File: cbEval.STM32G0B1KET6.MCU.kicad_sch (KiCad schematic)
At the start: 20 parts, among them J10 Bergstik-II_6, J11 Bergstik-II_6, J12 Bergstik-II_8, J13 Bergstik-II_6, J14 CNC-Tech 2x5, U1 STM32G0B1KET6, Y1 16.000MHz

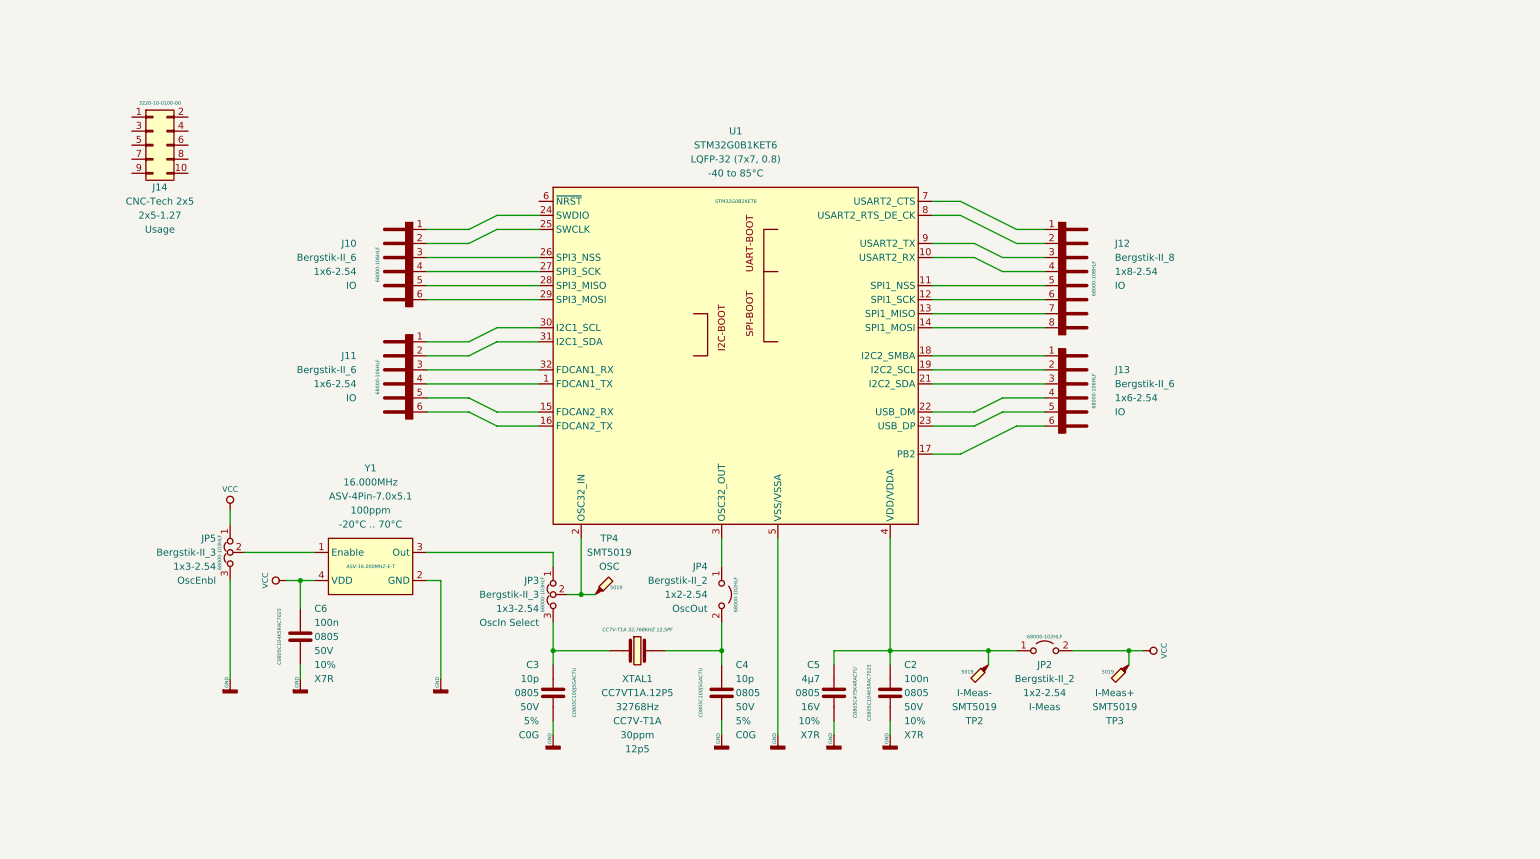
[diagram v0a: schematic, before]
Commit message: Zwischenstand (Sicherung)
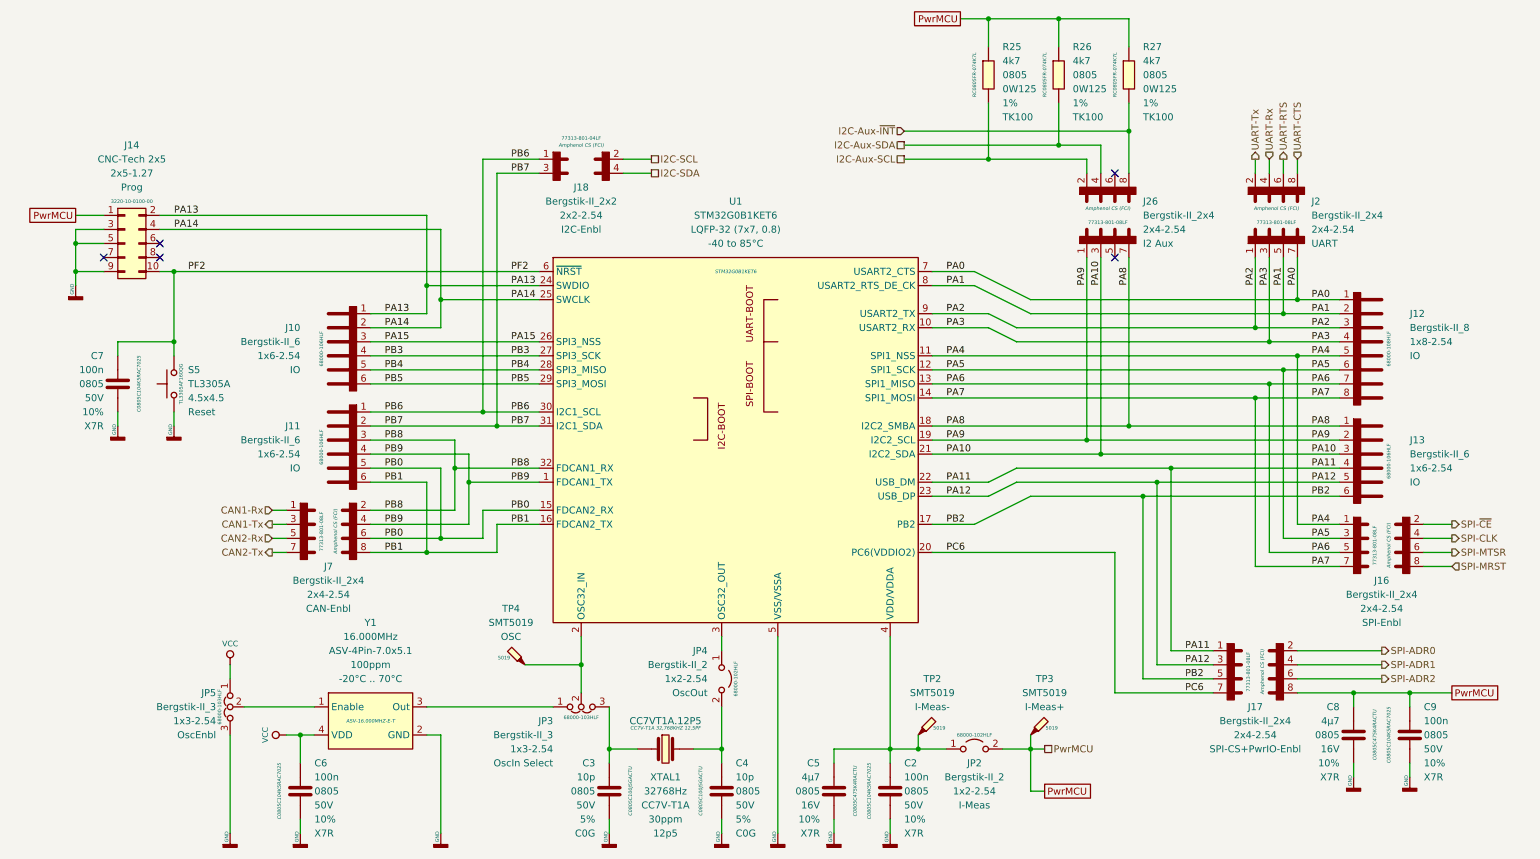
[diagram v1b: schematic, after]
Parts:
- added C7, C9: 100n, Capacitor_SMD:C_0805_2012Metric, symbol C.Kemet.MLCC.0805.X7R:100n
- added C8: 4µ7, Capacitor_SMD:C_0805_2012Metric, symbol C.Kemet.MLCC.0805.X7R:4µ7
- added J16, J17, J2, J26, J7: Bergstik-II_2x4, Connector_PinHeader_2.54mm:PinHeader_2x04_P2.54mm_Vertical, symbol J.PinHeader:Bergstik-II_2x4
- added J18: Bergstik-II_2x2, Connector_PinHeader_2.54mm:PinHeader_2x02_P2.54mm_Vertical, symbol J.PinHeader:Bergstik-II_2x2
- added R25, R26, R27: 4k7, Resistor_SMD:R_0805_2012Metric, symbol R.Yageo.RC0805:4k7
- added S5: TL3305A, Button_Switch_SMD:SW_SPST_TL3305A, symbol S:TL3305A
- J14: Usage Usage -> Prog
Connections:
- net GND: now also J14.3 (Pin_3), J14.5 (Pin_5), J14.9 (Pin_9), C7.2, C8.2, C9.2, S5.2
- net VCC: no longer JP2.2 (B), TP3.1
- net PA0: now reaches J12.1 (A1), U1.7 (USART2_CTS)
- net PA0: now also J2.7 (A4)
- net PA1: now reaches J12.2 (A2), U1.8 (USART2_RTS_DE_CK)
- net PA1: now also J2.5 (A3)
- net PA2: now reaches J12.3 (A3), U1.9 (USART2_TX)
- net PA2: now also J2.1 (A1)
- net PA3: now reaches J12.4 (A4), U1.10 (USART2_RX)
- net PA3: now also J2.3 (A2)
- net PA4: now reaches J12.5 (A5), U1.11 (SPI1_NSS)
- net PA4: now also J16.1 (A1)
- net PA5: now reaches J12.6 (A6), U1.12 (SPI1_SCK)
- net PA5: now also J16.3 (A2)
- net PA6: now reaches J12.7 (A7), U1.13 (SPI1_MISO)
- net PA6: now also J16.5 (A3)
- net PA7: now reaches J12.8 (A8), U1.14 (SPI1_MOSI)
- net PA7: now also J16.7 (A4)
- net PwrMCU: now reaches J14.1 (Pin_1)
- net PwrMCU: now also JP2.2 (B), TP3.1, C8.1, C9.1, J17.8 (B4), R25.1, R26.1, R27.1
- net PF2: now reaches J14.10 (Pin_10)
- net PF2: now also U1.6 (~{NRST}), C7.1, S5.1
- net PA13: now reaches J14.2 (Pin_2)
- net PA13: now also J10.1 (A1), U1.24 (SWDIO)
- net PA14: now reaches J14.4 (Pin_4)
- net PA14: now also J10.2 (A2), U1.25 (SWCLK)
- net PB9: now reaches J11.4 (A4), U1.1 (FDCAN1_TX)
- net PB9: now also J7.4 (B2)
- net PB0: now reaches J11.5 (A5), U1.15 (FDCAN2_RX)
- net PB0: now also J7.6 (B3)
- net PB1: now reaches J11.6 (A6), U1.16 (FDCAN2_TX)
- net PB1: now also J7.8 (B4)
- net PB2: now reaches J13.6 (A6), U1.17 (PB2)
- net PB2: now also J17.5 (A3)
- net PA8: now reaches J13.1 (A1), U1.18 (I2C2_SMBA)
- net PA8: now also J26.7 (A4)
- net PA9: now reaches J13.2 (A2), U1.19 (I2C2_SCL)
- net PA9: now also J26.1 (A1)
- net PA10: now reaches J13.3 (A3), U1.21 (I2C2_SDA)
- net PA10: now also J26.3 (A2)
- net PA11: now reaches J13.4 (A4), U1.22 (USB_DM)
- net PA11: now also J17.1 (A1)
- net PA12: now reaches J13.5 (A5), U1.23 (USB_DP)
- net PA12: now also J17.3 (A2)
- net PA15: now reaches J10.3 (A3), U1.26 (SPI3_NSS)
- net PB3: now reaches J10.4 (A4), U1.27 (SPI3_SCK)
- net PB4: now reaches J10.5 (A5), U1.28 (SPI3_MISO)
- net PB5: now reaches J10.6 (A6), U1.29 (SPI3_MOSI)
- net PB6: now reaches J11.1 (A1), U1.30 (I2C1_SCL)
- net PB6: now also J18.1 (A1)
- net PB7: now reaches J11.2 (A2), U1.31 (I2C1_SDA)
- net PB7: now also J18.3 (A2)
- net PB8: now reaches J11.3 (A3), U1.32 (FDCAN1_RX)
- net PB8: now also J7.2 (B1)
- new net CAN1-Rx: J7.1 (A1)
- new net CAN1-Tx: J7.3 (A2)
- new net CAN2-Rx: J7.5 (A3)
- new net CAN2-Tx: J7.7 (A4)
- new net I2C-Aux-SCL: J26.2 (B1), R25.2
- new net I2C-Aux-SDA: J26.4 (B2), R26.2
- new net I2C-Aux-~{INT}: J26.8 (B4), R27.2
- new net I2C-SCL: J18.2 (B1)
- new net I2C-SDA: J18.4 (B2)
- new net PC6: J17.7 (A4), U1.20 (PC6(VDDIO2))
- new net SPI-ADR0: J17.2 (B1)
- new net SPI-ADR1: J17.4 (B2)
- new net SPI-ADR2: J17.6 (B3)
- new net SPI-CLK: J16.4 (B2)
- new net SPI-MRST: J16.8 (B4)
- new net SPI-MTSR: J16.6 (B3)
- new net SPI-~{CE}: J16.2 (B1)
- new net UART-CTS: J2.8 (B4)
- new net UART-RTS: J2.6 (B3)
- new net UART-Rx: J2.4 (B2)
- new net UART-Tx: J2.2 (B1)
- no-connect marks 0 -> 5
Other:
- moved on the sheet: C2, C3, C4, C5, C6, J10, J11, J12, J13, J14, JP2, JP3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
